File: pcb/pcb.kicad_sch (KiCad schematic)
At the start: 57 parts, among them J1 USB_C_Receptacle_USB2.0_16P, J2 Conn_01x02, K1 SW_Push, K10 SW_Push, K11 SW_Push, K12 SW_Push, K13 SW_Push, K14 SW_Push, K15 SW_Push, K16 SW_Push, K17 SW_Push, K18 SW_Push, K19 SW_Push, K2 SW_Push, K20 SW_Push, K21 SW_Push, K3 SW_Push, K4 SW_Push, K5 SW_Push, K6 SW_Push, K7 SW_Push, K8 SW_Push, K9 SW_Push, U1 SRV05-4, U2 ProMicro, U3 SRV05-4

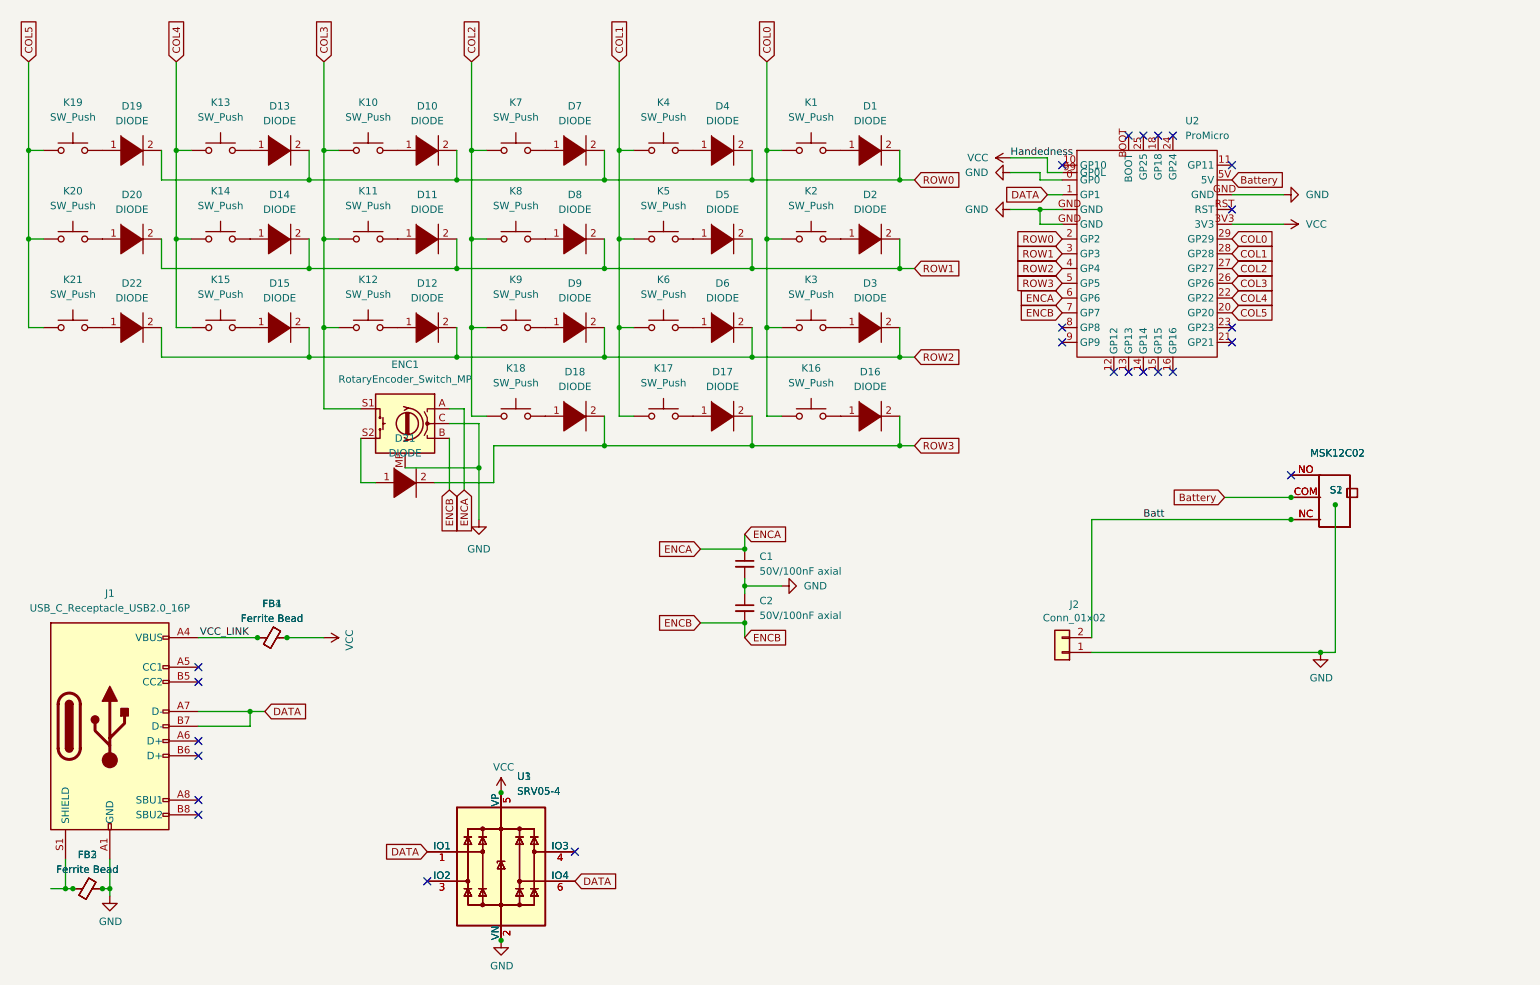
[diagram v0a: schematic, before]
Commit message: cirrus40, second manufactured version
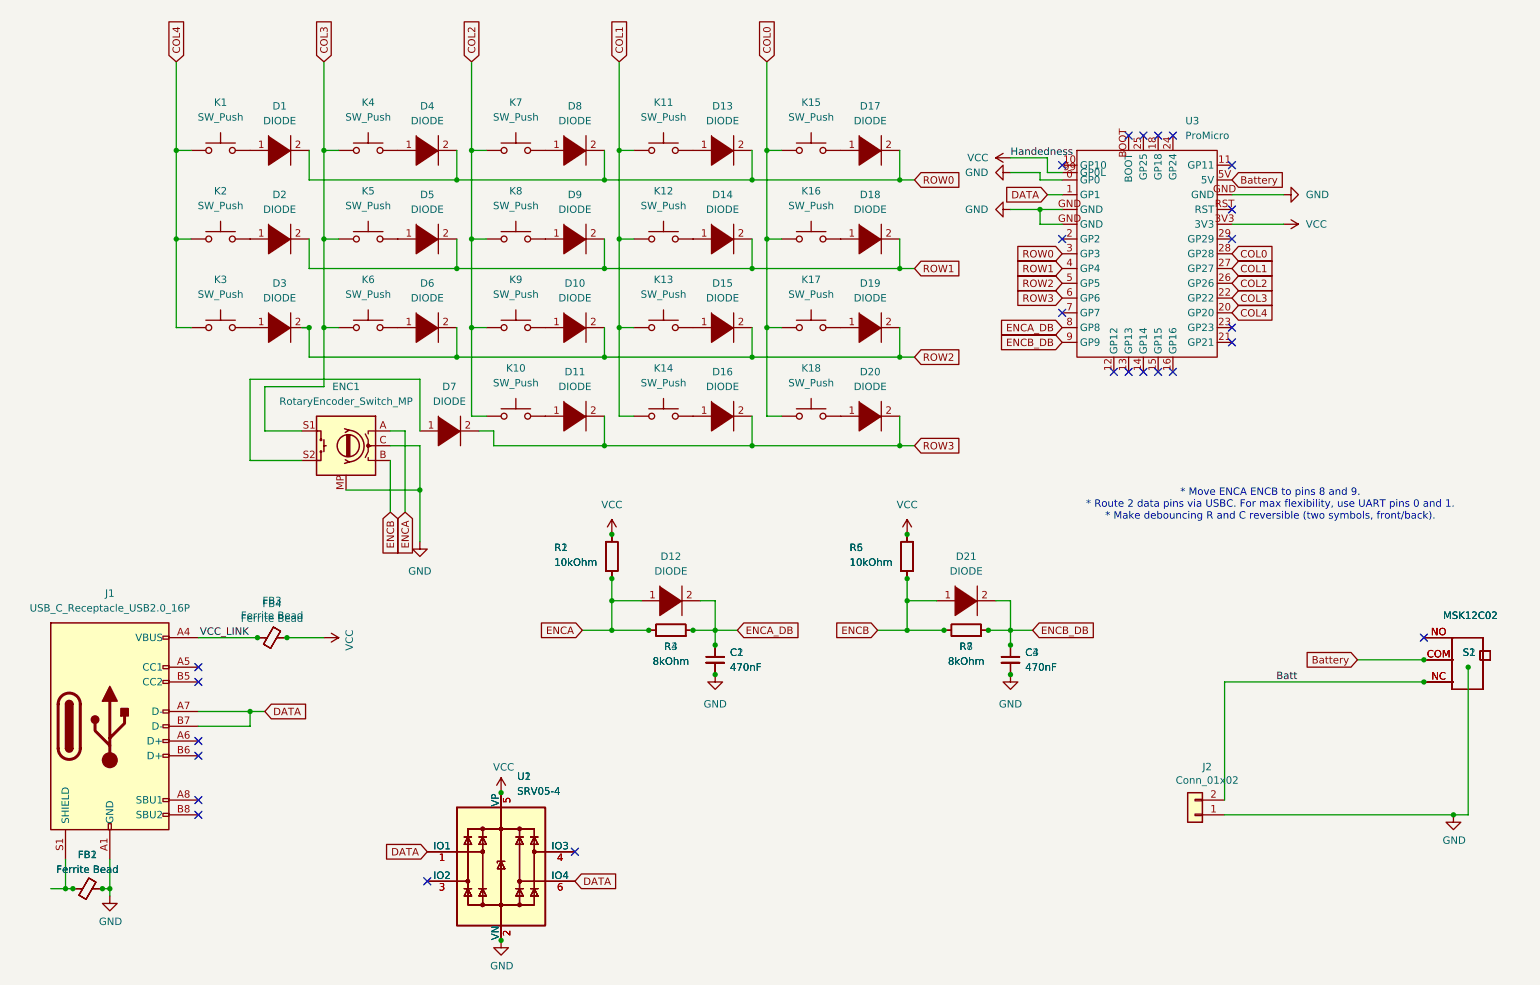
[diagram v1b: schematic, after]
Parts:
- removed D19, D20, D22: DIODE, footprints:Diode-dual, symbol cirrus40:DIODE
- removed K19, K20, K21: SW_Push, footprints:SW_MX_HotSwap_Reversible, symbol cirrus40:SW_Push
- added C1, C3: 470nF, Capacitor_SMD:C_0805_2012Metric_Pad1.18x1.45mm_HandSolder, symbol cirrus40:C_Small
- added D12, D21: DIODE, footprints:Diode-dual, symbol cirrus40:DIODE
- added R1, R2, R5, R6: 10kOhm, Resistor_SMD:R_0805_2012Metric_Pad1.20x1.40mm_HandSolder, symbol Device:R
- added R3, R4, R7, R8: 8kOhm, Resistor_SMD:R_0805_2012Metric_Pad1.20x1.40mm_HandSolder, symbol Device:R
- C2: renamed from C1; value 50V/100nF axial -> 470nF; footprint footprints:RESISTOR_Reversible -> Capacitor_SMD:C_0805_2012Metric_Pad1.18x1.45mm_HandSolder
- C4: renamed from C2; value 50V/100nF axial -> 470nF; footprint footprints:RESISTOR_Reversible -> Capacitor_SMD:C_0805_2012Metric_Pad1.18x1.45mm_HandSolder
- FB1: renamed from FB2; footprint footprints:C_0603_1608Metric_Pad1.08x0.95mm_HandSolder -> Capacitor_SMD:C_0805_2012Metric_Pad1.18x1.45mm_HandSolder
- FB2: renamed from FB3; footprint footprints:C_0603_1608Metric_Pad1.08x0.95mm_HandSolder -> Capacitor_SMD:C_0805_2012Metric_Pad1.18x1.45mm_HandSolder
- FB3: renamed from FB4; footprint footprints:C_0603_1608Metric_Pad1.08x0.95mm_HandSolder -> Capacitor_SMD:C_0805_2012Metric_Pad1.18x1.45mm_HandSolder
- FB4: renamed from FB1; footprint footprints:C_0603_1608Metric_Pad1.08x0.95mm_HandSolder -> Capacitor_SMD:C_0805_2012Metric_Pad1.18x1.45mm_HandSolder
- renumbered D13 to D1, D9 to D10, D18 to D11, D4 to D13, D5 to D14, D6 to D15, D17 to D16, D1 to D17, D2 to D18, D3 to D19, D14 to D2, D16 to D20, D15 to D3, D10 to D4, D11 to D5, D12 to D6, D21 to D7, D7 to D8, D8 to D9, K13 to K1, K18 to K10, K4 to K11, K5 to K12, K6 to K13, K17 to K14, K1 to K15, K2 to K16, K3 to K17, K16 to K18, K14 to K2, K15 to K3, K10 to K4, K11 to K5, K12 to K6, U3 to U1, U1 to U2, U2 to U3
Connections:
- net COL5 is gone; now on net COL4: U3.20 (GP20)
- net COL0: now also U3.28 (GP28); no longer U3.29 (GP29)
- net COL1: now also U3.27 (GP27); no longer U3.28 (GP28)
- net COL2: now also U3.26 (GP26); no longer U3.27 (GP27)
- net COL3: now also U3.22 (GP22); no longer U3.26 (GP26)
- net COL4: no longer U3.22 (GP22)
- net ENCA: now also D12.1 (K), R1.2, R2.2, R3.1, R4.1; no longer C2.1, U3.6 (GP6)
- net ENCB: now also D21.1 (K), R5.2, R6.2, R7.1, R8.1; no longer C4.2, U3.7 (GP7)
- net GND: now also C4.2, C1.2, C3.2; no longer C4.1
- net ROW0: now also U3.3 (GP3); no longer U3.2 (GP2)
- net ROW1: now also U3.4 (GP4); no longer U3.3 (GP3)
- net ROW2: now also U3.5 (GP5); no longer U3.4 (GP4)
- net ROW3: now also U3.6 (GP6); no longer U3.5 (GP5)
- net VCC: now also R1.1, R2.1, R5.1, R6.1
- net ENCA_DB: now reaches U3.8 (GP8)
- net ENCA_DB: now also C2.1, C1.1, D12.2 (A), R3.2, R4.2
- net ENCB_DB: now reaches U3.9 (GP9)
- net ENCB_DB: now also C4.1, C3.1, D21.2 (A), R7.2, R8.2
- no-connect marks 25 -> 26
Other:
- note added: "* Move ENCA ENCB to pins 8 and 9. * Route 2 data pins via USBC. For max flexibility, use UART pins 0 and 1. * Make debouncing R and C reversible (two symbols, front/back)."
- moved on the sheet: C2, C4, D7, ENC1, J2, S1, S2
